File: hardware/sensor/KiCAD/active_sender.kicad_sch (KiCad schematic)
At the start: 24 parts, among them J1 USB-C input, J2 Buzzer, J3 Water Sensor, Q1 AO3400A, SW1 SW_Push, SW2 SW_SPDT, U1 ESP32-C3_SUPERMINI_TH, U2 Ai-Thinker-Ra-02, U3 AMS1117-3.3

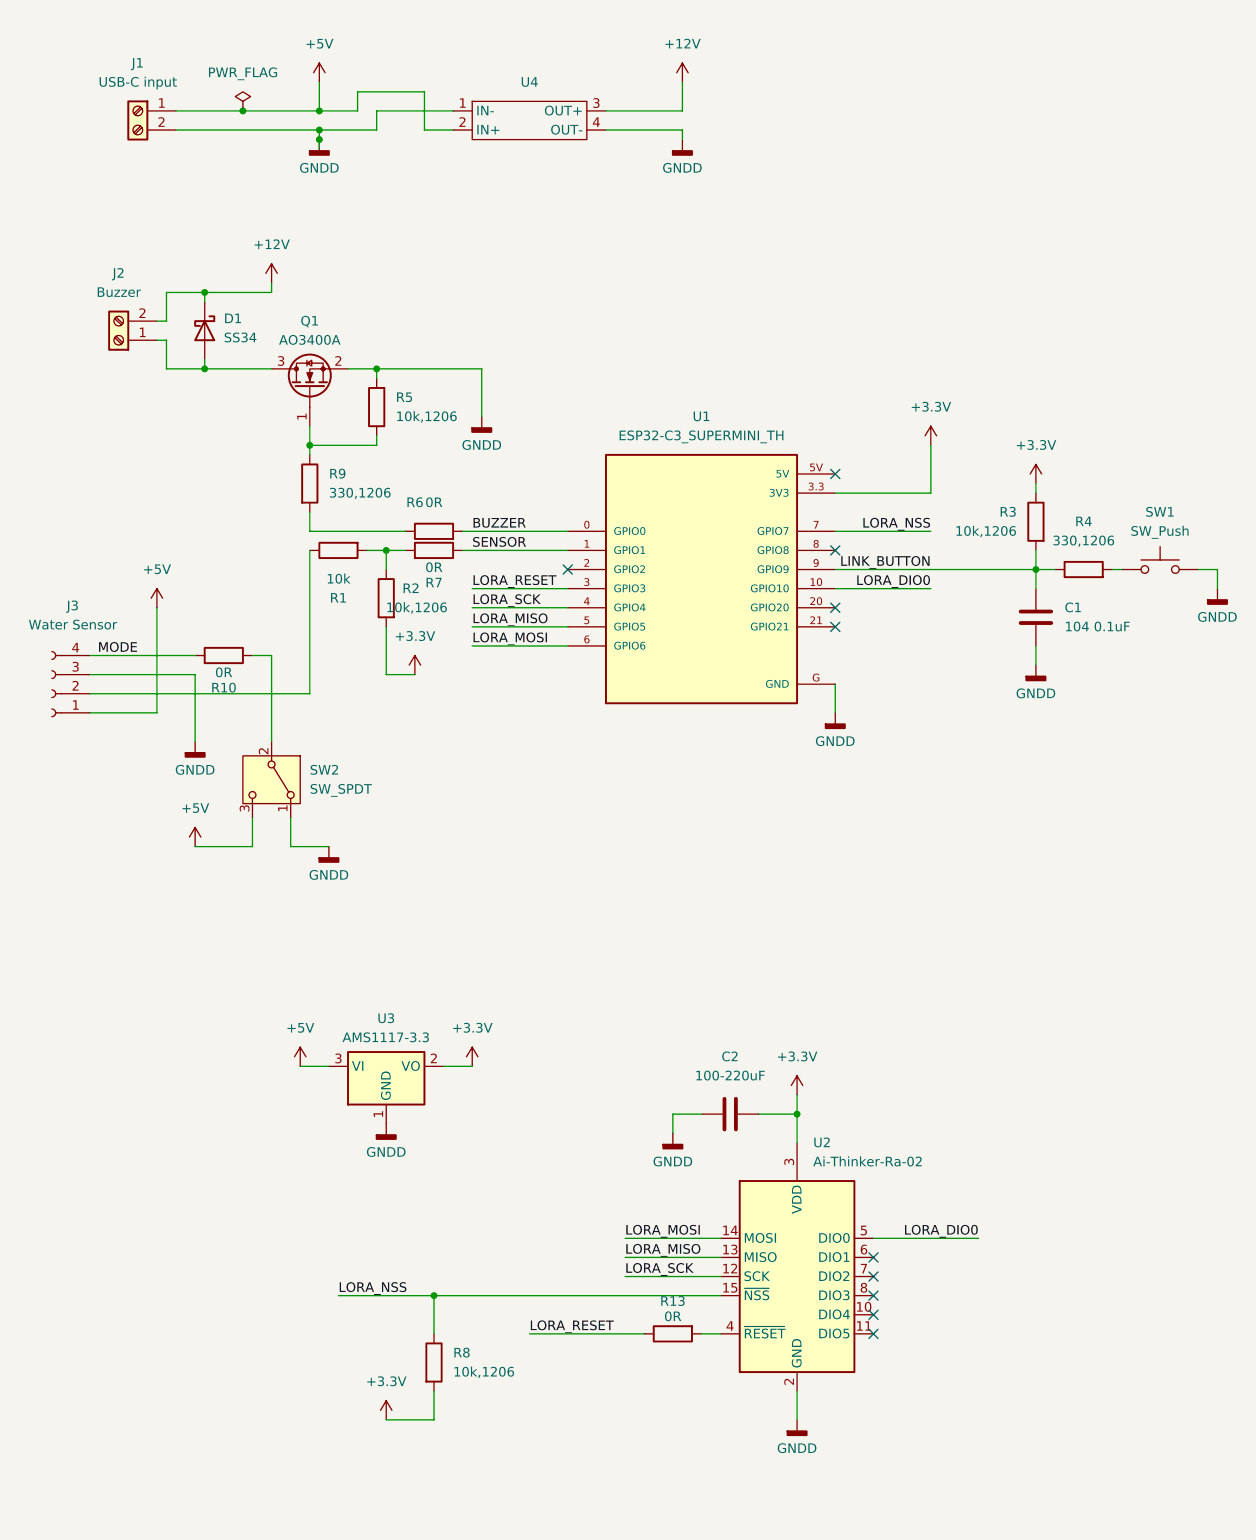
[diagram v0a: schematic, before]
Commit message: dev
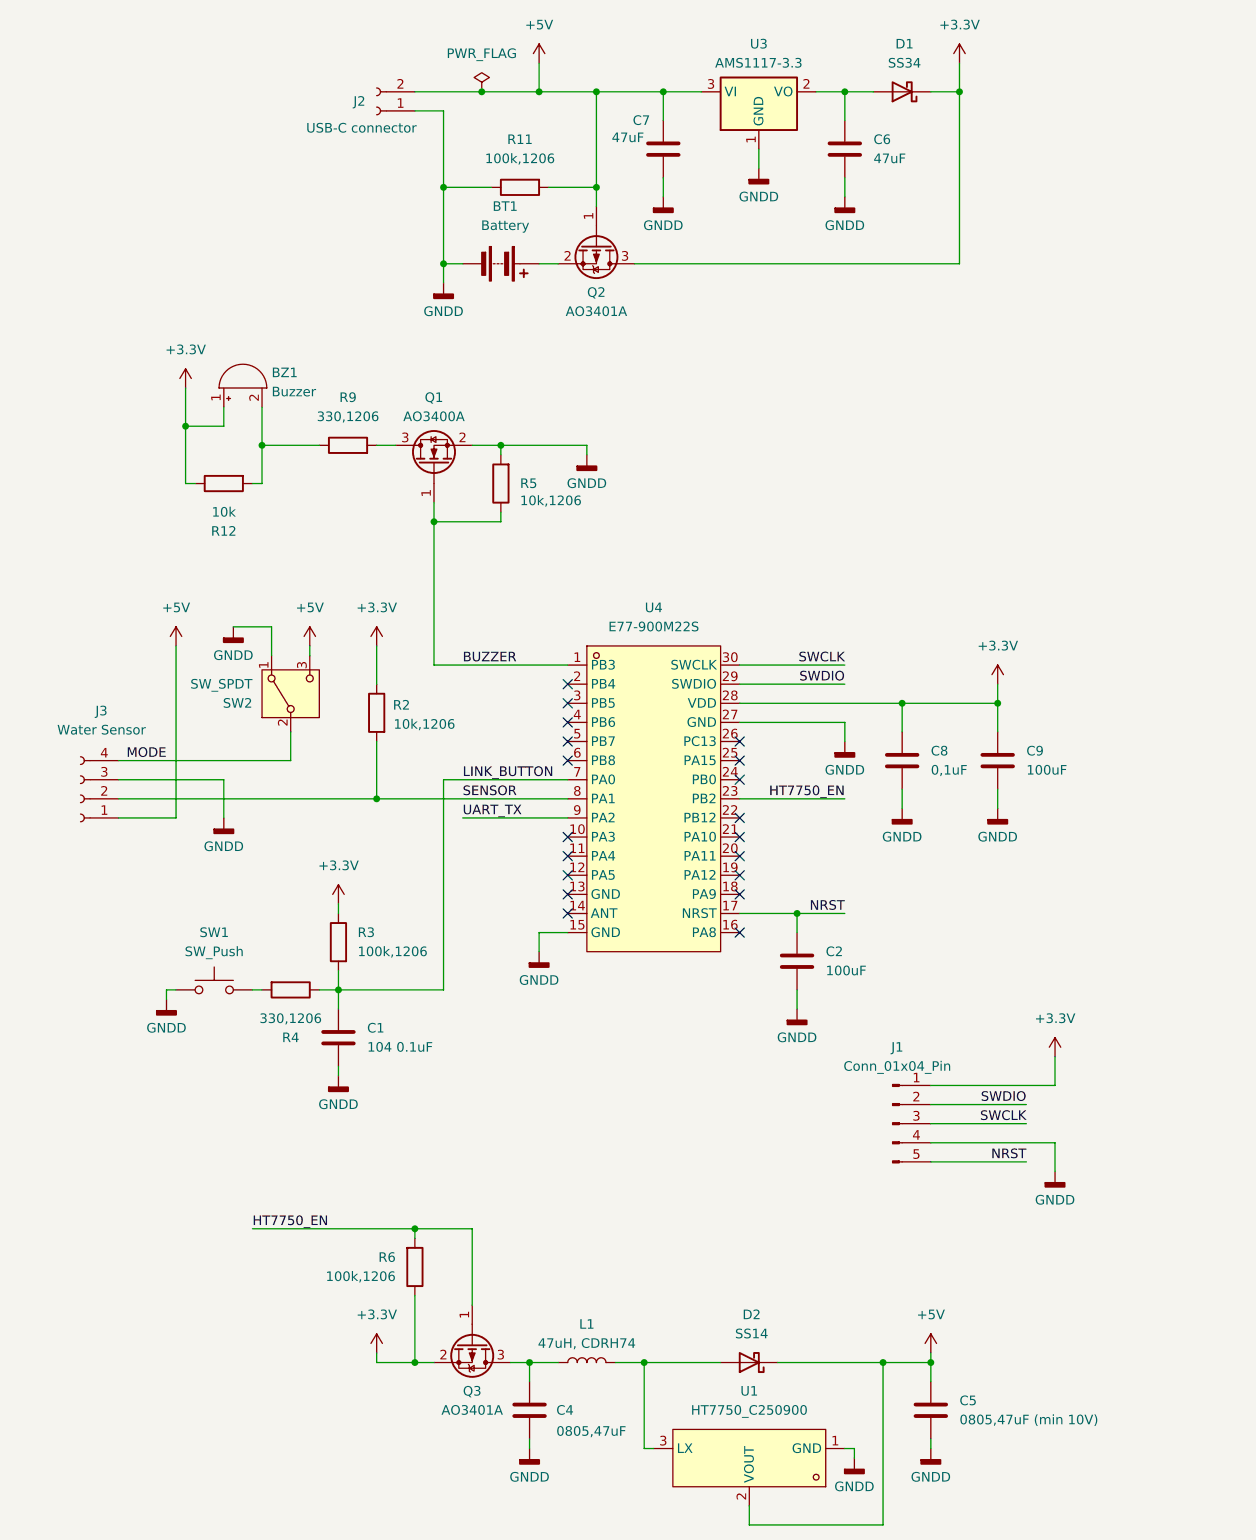
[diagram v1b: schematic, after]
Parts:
- removed J1: USB-C input, TerminalBlock_Phoenix:TerminalBlock_Phoenix_MKDS-1,5-2_1x02_P5.00mm_Horizontal, symbol Connector:Screw_Terminal_01x02
- removed J2: Buzzer, TerminalBlock_Phoenix:TerminalBlock_Phoenix_MKDS-1,5-2_1x02_P5.00mm_Horizontal, symbol Connector:Screw_Terminal_01x02
- removed R1: 10k, Resistor_SMD:R_1206_3216Metric_Pad1.30x1.75mm_HandSolder, symbol Device:R
- removed R10, R13, R7: 0R, Resistor_SMD:R_2512_6332Metric_Pad1.40x3.35mm_HandSolder, symbol Device:R
- removed R8: 10k,1206, Resistor_SMD:R_1206_3216Metric_Pad1.30x1.75mm_HandSolder, symbol Device:R
- removed U1: ESP32-C3_SUPERMINI_TH, custom_footprints:MODULE_ESP32-C3_SUPERMINI_TH, symbol Custom_library:ESP32-C3_SUPERMINI_TH
- removed U2: Ai-Thinker-Ra-02, custom_footprints:Ai-Thinker-Ra-01-LoRa BREAKOUT BOARD, symbol RF_Module:Ai-Thinker-Ra-02
- removed U4: (no value), custom_footprints:CKCS BS-01, symbol Custom_library:CKCS_BS-01
- added BT1: Battery, custom_footprints:BHC-CR123A, symbol Device:Battery
- added BZ1: Buzzer, Buzzer_Beeper:Buzzer_12x9.5RM7.6, symbol Device:Buzzer
- added C4: 0805,47uF, Capacitor_SMD:C_0805_2012Metric_Pad1.18x1.45mm_HandSolder, symbol Device:C
- added C5: 0805,47uF (min 10V), Capacitor_SMD:C_0805_2012Metric_Pad1.18x1.45mm_HandSolder, symbol Device:C
- added C6, C7: 47uF, Capacitor_SMD:C_0805_2012Metric_Pad1.18x1.45mm_HandSolder, symbol Device:C
- added C8: 0,1uF, Capacitor_SMD:C_0805_2012Metric_Pad1.18x1.45mm_HandSolder, symbol Device:C
- added C9: 100uF, Capacitor_SMD:C_0805_2012Metric_Pad1.18x1.45mm_HandSolder, symbol Device:C
- added D2: SS14, Diode_SMD:D_SMA, symbol Diode:SS14
- added J1: Conn_01x04_Pin, Connector_PinHeader_2.00mm:PinHeader_1x05_P2.00mm_Vertical, symbol Connector:Conn_01x05_Pin
- added J2: USB-C connector, Connector_JST:JST_PH_B2B-PH-K_1x02_P2.00mm_Vertical, symbol Connector:Conn_01x02_Socket
- added L1: 47uH, CDRH74, Inductor_SMD:L_7.3x7.3_H4.5, symbol Device:L
- added Q2, Q3: AO3401A, Package_TO_SOT_SMD:SOT-23, symbol Transistor_FET:AO3401A
- added R11: 100k,1206, Resistor_SMD:R_1206_3216Metric_Pad1.30x1.75mm_HandSolder, symbol Device:R
- added R12: 10k, Resistor_SMD:R_1206_3216Metric_Pad1.30x1.75mm_HandSolder, symbol Device:R
- added U1: HT7750_C250900, custom_footprints:HT7750, symbol Custom_library:HT7750_C250900
- added U4: E77-900M22S, custom_footprints:COMM-SMD_30P-L20.0-W14.0-P1.27, symbol Custom_library:E77-900M22S
- C2: value 100-220uF -> 100uF; footprint Capacitor_SMD:C_Elec_5x5.4 -> Capacitor_SMD:C_0805_2012Metric_Pad1.18x1.45mm_HandSolder
- R3: value 10k,1206 -> 100k,1206
- R6: value 0R -> 100k,1206; footprint Resistor_SMD:R_2512_6332Metric_Pad1.40x3.35mm_HandSolder -> Resistor_SMD:R_1206_3216Metric_Pad1.30x1.75mm_HandSolder
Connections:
- net +12V is gone; now on net +3.3V: D1.1 (K)
- net +3.3V: now also R2.1, R6.1, BZ1.1 (+), C8.1, C9.1, J1.1 (Pin_1), Q2.3 (D), Q3.2 (S), R12.1, U4.28 (VDD); no longer C2.2, R2.2, U3.2 (VO)
- net +5V: now also C5.1, C7.1, D2.1 (K), J2.2 (Pin_2), Q2.1 (G), R11.2, U1.2 (VOUT)
- net BUZZER: now also Q1.1 (G), R5.1, U4.1 (PB3); no longer R6.2
- net GNDD: now also C2.2, SW1.1, BT1.2 (-), C4.2, C5.2, C6.2, C7.2, C8.2, C9.2, J1.4 (Pin_4), J2.1 (Pin_1), R11.1, U1.1 (GND), U4.15 (GND), U4.27 (GND); no longer C2.1, SW1.2
- net LINK_BUTTON: now also U4.7 (PA0)
- net MODE: now also SW2.2 (B)
- net SENSOR: now also J3.2 (Pin_2), R2.2, U4.8 (PA1)
- net at R9.2: now also Q1.3 (D); no longer R6.1
- net at R4.2: now also SW1.2; no longer SW1.1
- net at D1.2 (A): now also U3.2 (VO), C6.1; no longer Q1.3 (D)
- new net: BZ1.2 (-), R12.2, R9.1
- new net: C4.1, L1.1, Q3.3 (D)
- new net: D2.2 (A), L1.2, U1.3 (LX)
- new net: BT1.1 (+), Q2.2 (S)
- new net HT7750_EN: Q3.1 (G), R6.2, U4.23 (PB2)
- new net NRST: C2.1, J1.5 (Pin_5), U4.17 (NRST)
- new net SWCLK: J1.3 (Pin_3), U4.30 (SWCLK)
- new net SWDIO: J1.2 (Pin_2), U4.29 (SWDIO)
- new net UART_TX: U4.9 (PA2)
- no-connect marks 10 -> 19
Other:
- moved on the sheet: C1, J3, Q1, R2, R3, R4, R5, SW1, SW2, U3
